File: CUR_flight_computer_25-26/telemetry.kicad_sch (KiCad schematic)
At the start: 19 parts, among them J14 Conn_Coaxial_Small, U5 E22-400MM_22S

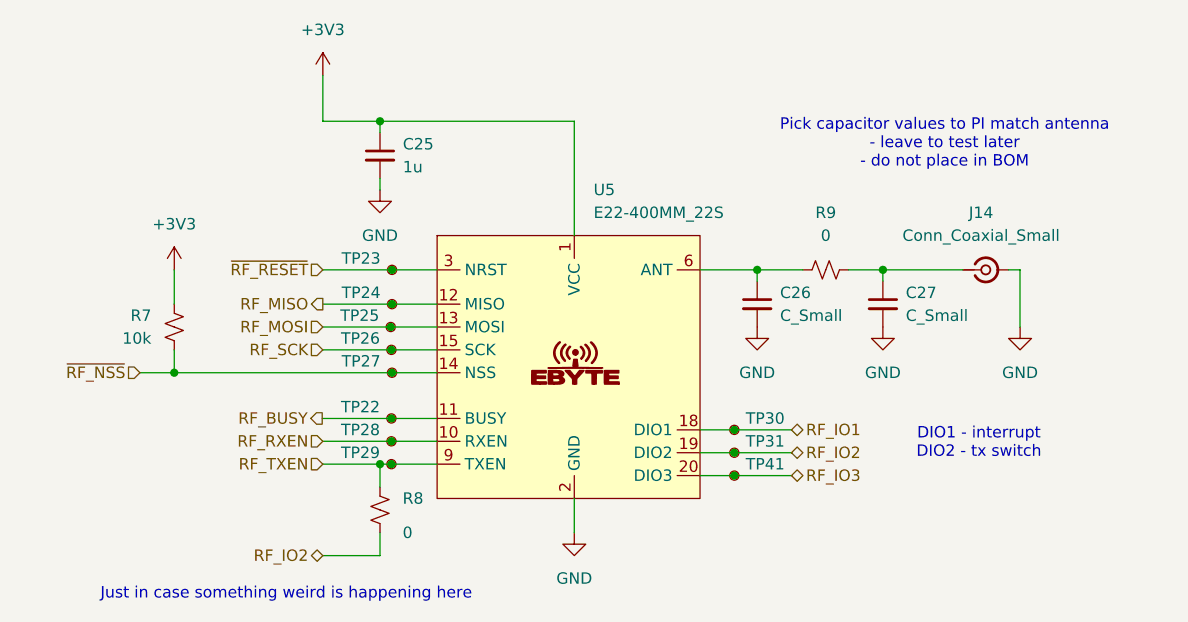
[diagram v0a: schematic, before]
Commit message: Update telemetry.kicad_sch
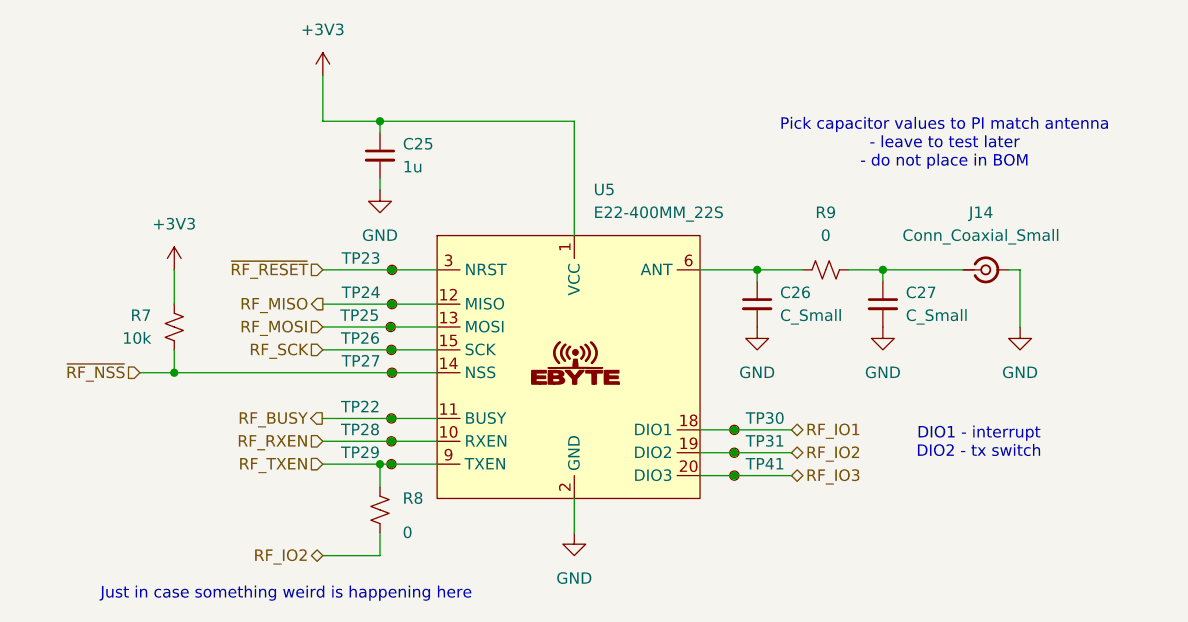
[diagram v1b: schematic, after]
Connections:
- net RF_BUSY: now also U5.11 (BUSY)
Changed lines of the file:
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@@
 	(wire
 		(pts
-			(xy 64.77 66.04) (xy 69.7821 66.04)
+			(xy 64.77 66.04) (xy 69.85 66.04)
 		)
 		(stroke
